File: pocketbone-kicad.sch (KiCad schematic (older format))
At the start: 62 parts, among them P1 USB_OTG, P2 USB_OTG, P3 CONN_01X10, P4 CONN_02X02, SW1 SW_PUSH_SMALL_H, SW2 SW_PUSH_SMALL_H, U1 SN74LVC1G07, U2 OSD3358, U3 24LC32AT-I/OT, U4 TPS2051C, Y2 24MHz

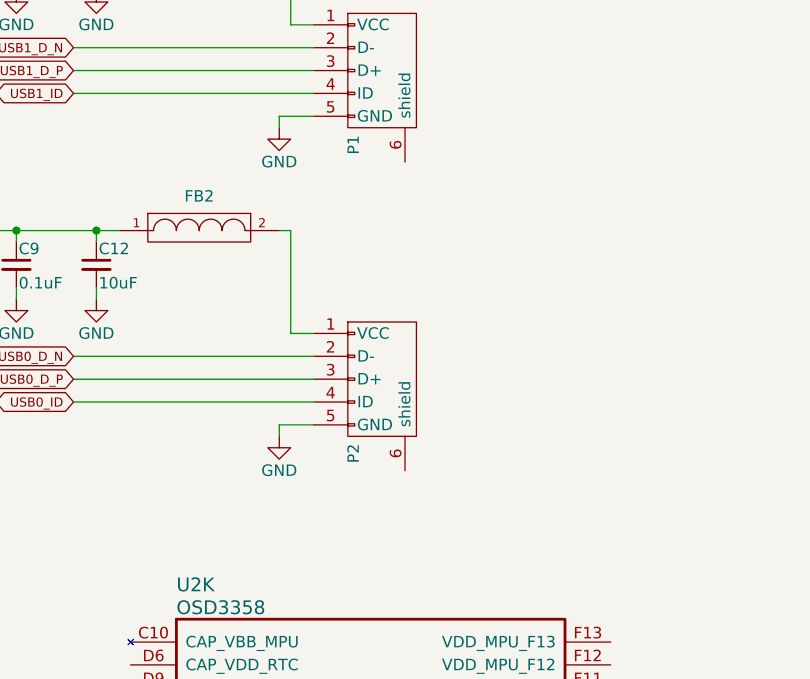
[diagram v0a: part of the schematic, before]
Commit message: Last minute tweaks
This version is posted to OSHpark site for anyone to order.
Order at your own risk.

Signed-off-by: Michael Welling <mwelling@ieee.org>
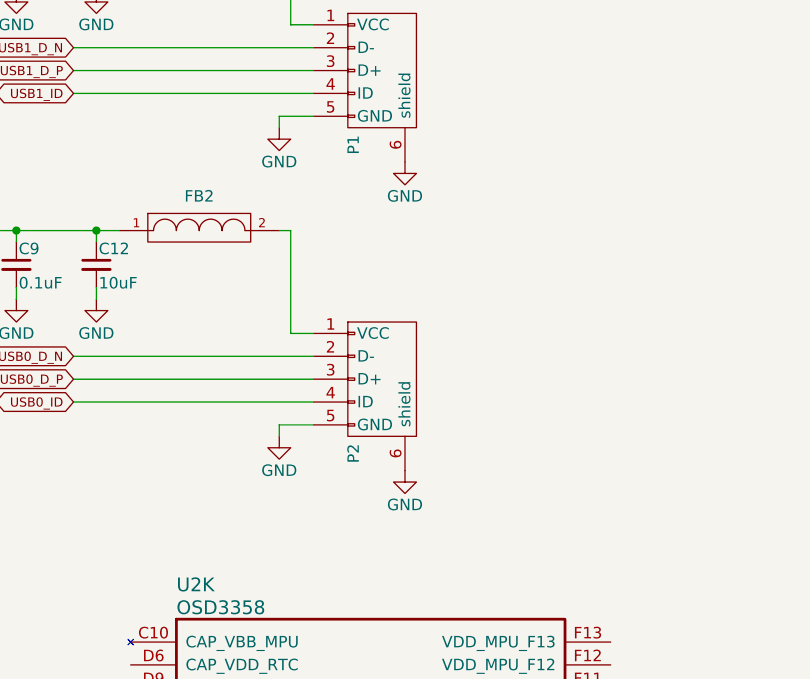
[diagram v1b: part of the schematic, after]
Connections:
- net GND: now also P1.6 (shield), P2.6 (shield)
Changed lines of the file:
@@
 Wire Wire Line
 	2400 2250 2400 2350
+$Comp
+L GND #PWR?
+U 1 1 589CA027
+P 9800 11250
+F 0 "#PWR?" H 9800 11000 50  0001 C CNN
+F 1 "GND" H 9800 11100 50  0000 C CNN
+F 2 "" H 9800 11250 50  0000 C CNN
+F 3 "" H 9800 11250 50  0000 C CNN
+	1    9800 11250
+	1    0    0    -1
+$EndComp
+$Comp
+L GND #PWR?
+U 1 1 589CA10D
+P 9800 9900
+F 0 "#PWR?" H 9800 9650 50  0001 C CNN
+F 1 "GND" H 9800 9750 50  0000 C CNN
+F 2 "" H 9800 9900 50  0000 C CNN
+F 3 "" H 9800 9900 50  0000 C CNN
+	1    9800 9900
+	1    0    0    -1
+$EndComp
 $EndSCHEMATC
